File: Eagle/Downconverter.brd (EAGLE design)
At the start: 40 x 40 mm, 26 parts, among them J2 3.5HEADPHONEJACK, J5 U.FL_CONN, J6 U.FL_CONN, U1 5V_REG, U2 MIXER, U3 DUAL_OP_AMP_LMV822, U4 DIGITAL_POTDIGITAL_POT

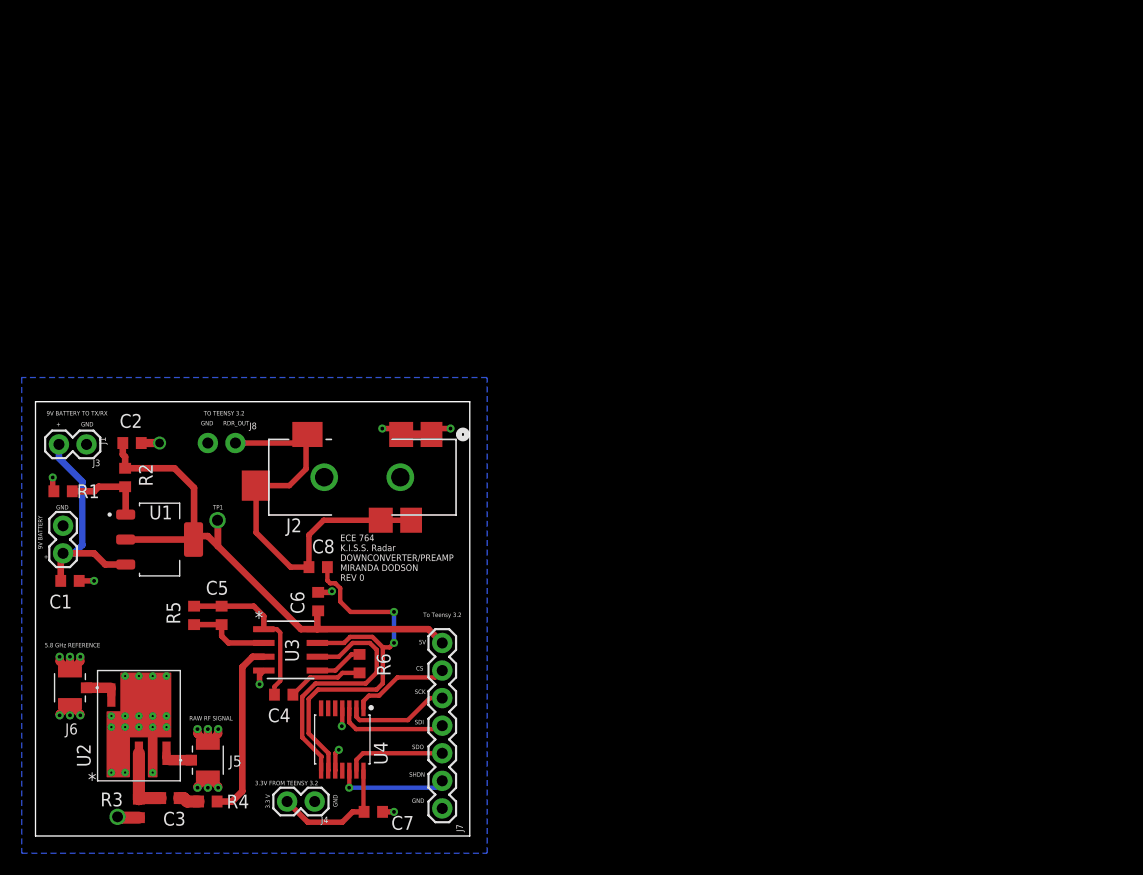
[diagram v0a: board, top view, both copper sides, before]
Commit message: update
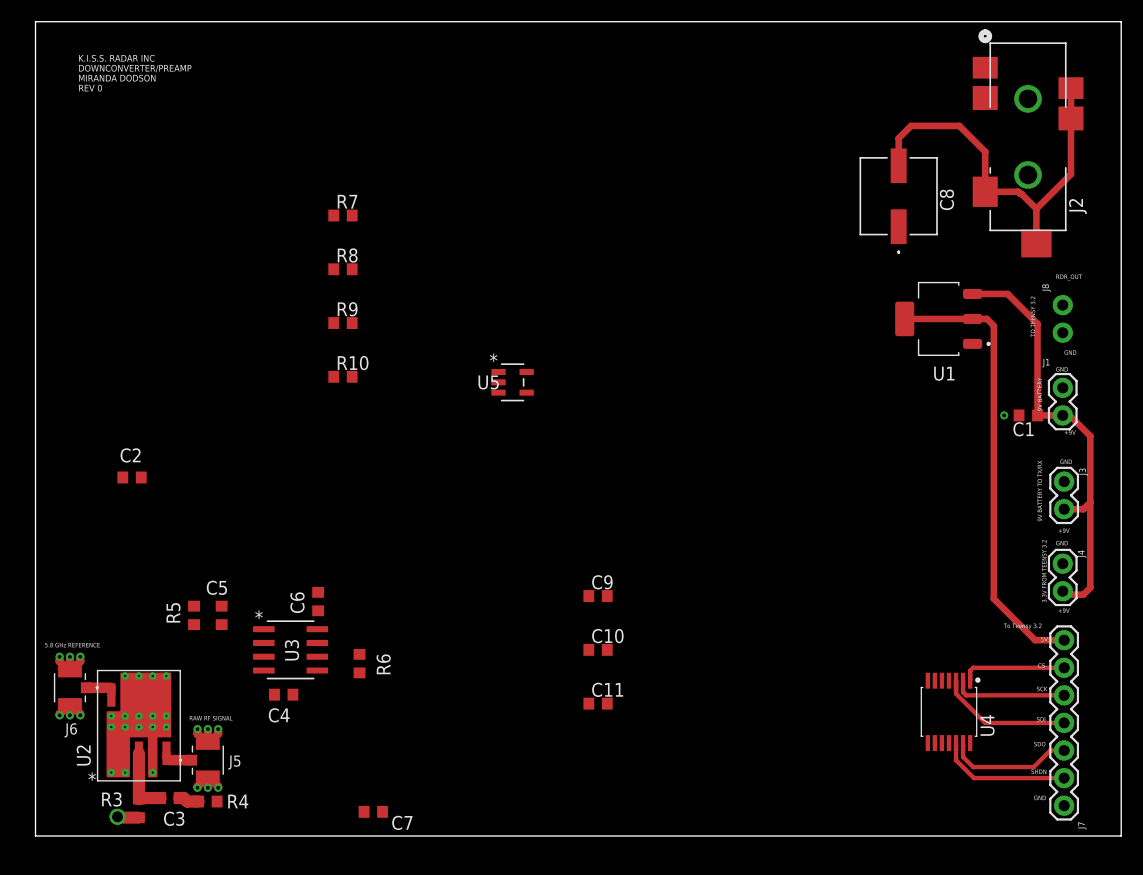
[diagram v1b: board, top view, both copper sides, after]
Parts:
- removed R1: 330, 764Library:R0603
- removed R2: 110, 764Library:R0603
- added C10: 100uF, 764Library:R0603
- added C11: 470pF, 764Library:R0603
- added C9: 10uF, 764Library:R0603
- added R10, R7, R8, R9: 1k, 764Library:R0603
- added U5: TC1185-3.3VCT713, 764Library:SOT-23-5_MC
- C3, C4: value 1uF -> 5.6uF
- C8: value 1uF -> 100uF; device 764Library:R0603 -> 764Library:EXV-9G
- moved J1 92.9 mm to (94.6, 41.3)
- moved J3 90.1 mm to (94.7, 32.6), turned to 270 degrees
- moved C1 89.6 mm to (91.4, 38.7), turned to 180 degrees
- moved J8 77.3 mm to (94.6, 48.9), turned to 270 degrees
- moved J2 74.8 mm to (95.4, 63.0), turned to 270 degrees
- moved U1 74.6 mm to (83.2, 47.6), turned to 90 degrees
- moved J4 72.3 mm to (94.6, 25.1), turned to 270 degrees
- moved C8 63.4 mm to (79.5, 58.9), turned to 90 degrees
- moved J7 57.3 mm to (94.7, 2.79)
- moved U4 55.9 mm to (84.1, 11.4)
- moved C2 3.17 mm to (8.89, 33.0)
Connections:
- removed net N$1: R1.2, R2.1, U1.1
- removed net N$12: C8.1, U3.7, U4.9
- new net AUDIO_OUTPUT: C8.2, J2.3, J2.4, J2.7, J2.8
- new net N$5: C11.1, U5.4
- net 3.3V: now also C10.1, C6.1, R10.1, R7.1, U3.8, U5.5; no longer J4.2
- net 5V: now also C9.1, U5.1, U5.3; no longer C6.1, R2.2, U3.8
- net 9V: now also J4.2
- net GND: now also C10.2, C11.2, C9.2, R8.2, R9.2, U1.1, U5.2; no longer R1.1
- net N$4: now also R7.2, R8.1
- net N$8: now also R10.2, R9.1
- net RDR_OUT: now also C8.1, U3.7, U4.9; no longer C8.2, J2.3, J2.4, J2.7, J2.8
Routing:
- net RDR_OUT: track 38.5 -> 0.04 mm
- net N$12: track 38.1 -> 0.00 mm, vias 2 -> 0
- net AUDIO_OUTPUT: track 0.00 -> 36.6 mm
- net N$13: track 23.7 -> 0.00 mm
- net 9V: track 21.1 -> 40.8 mm
- net GND: track 45.3 -> 25.9 mm, vias 23 -> 14
- net N$4: track 16.5 -> 0.00 mm
- net N$6: track 15.6 -> 0.00 mm
- net 3.3V: track 12.5 -> 0.19 mm
- net 5V: track 51.8 -> 41.7 mm, vias 1 -> 0
- net N$9: track 7.74 -> 0.00 mm
- net N$1: track 7.62 -> 0.00 mm
- net N$7: track 7.18 -> 0.21 mm
- net N$8: track 4.50 -> 0.10 mm
- net SDI: track 10.3 -> 13.2 mm
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- removed copper zone on layer 16, net GND
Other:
- board size 40 x 40 mm -> 100 x 75 mm
- board text added: "+9V"
- board text added: "K.I.S.S. RADAR INC DOWNCONVERTER/PREAMP MIRANDA DODSON REV 0"
- board text removed: "+"
- board text removed: "3.3 V"
- board text removed: "ECE 764 K.I.S.S. Radar DOWNCONVERTER/PREAMP MIRANDA DODSON REV 0"
- board text removed: "TP1"
